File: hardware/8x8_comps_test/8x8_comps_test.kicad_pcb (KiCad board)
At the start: 2 copper layers, 47.8 x 47.5 mm, 24 parts

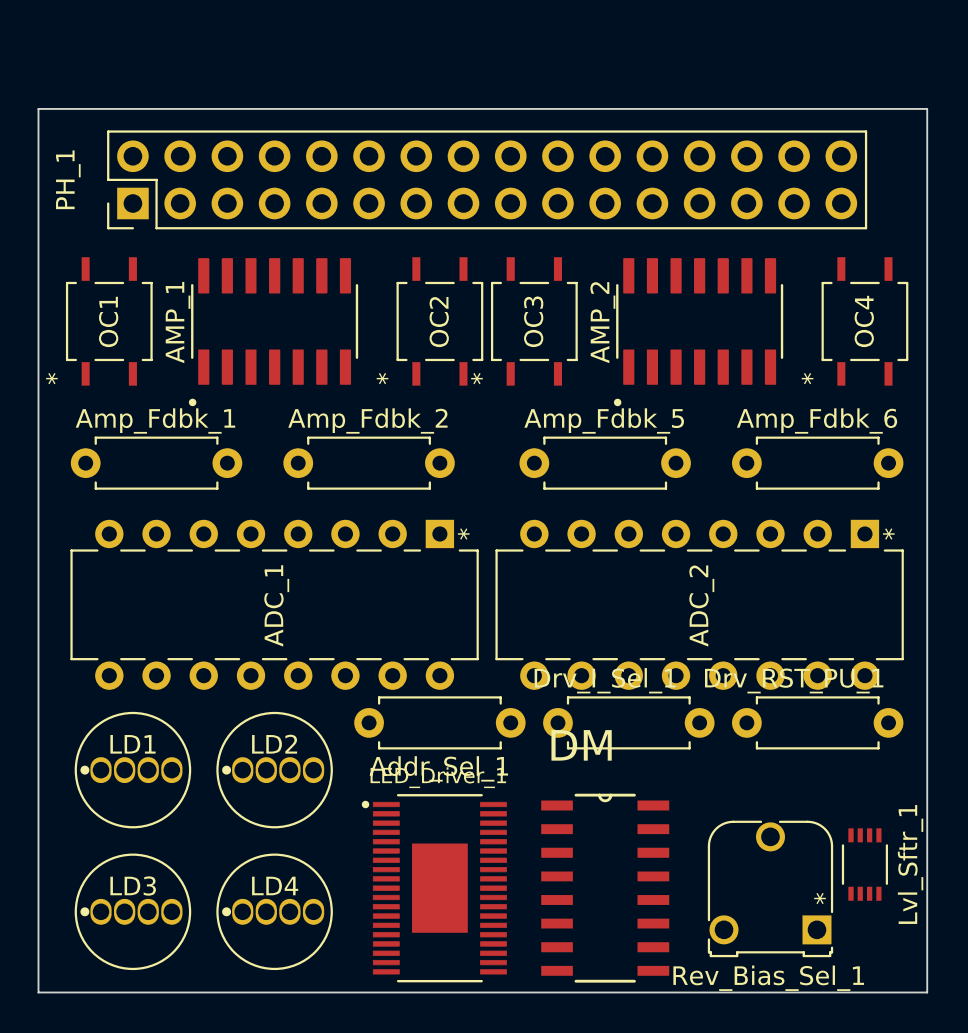
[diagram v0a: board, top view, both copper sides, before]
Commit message: Changed Test Layout
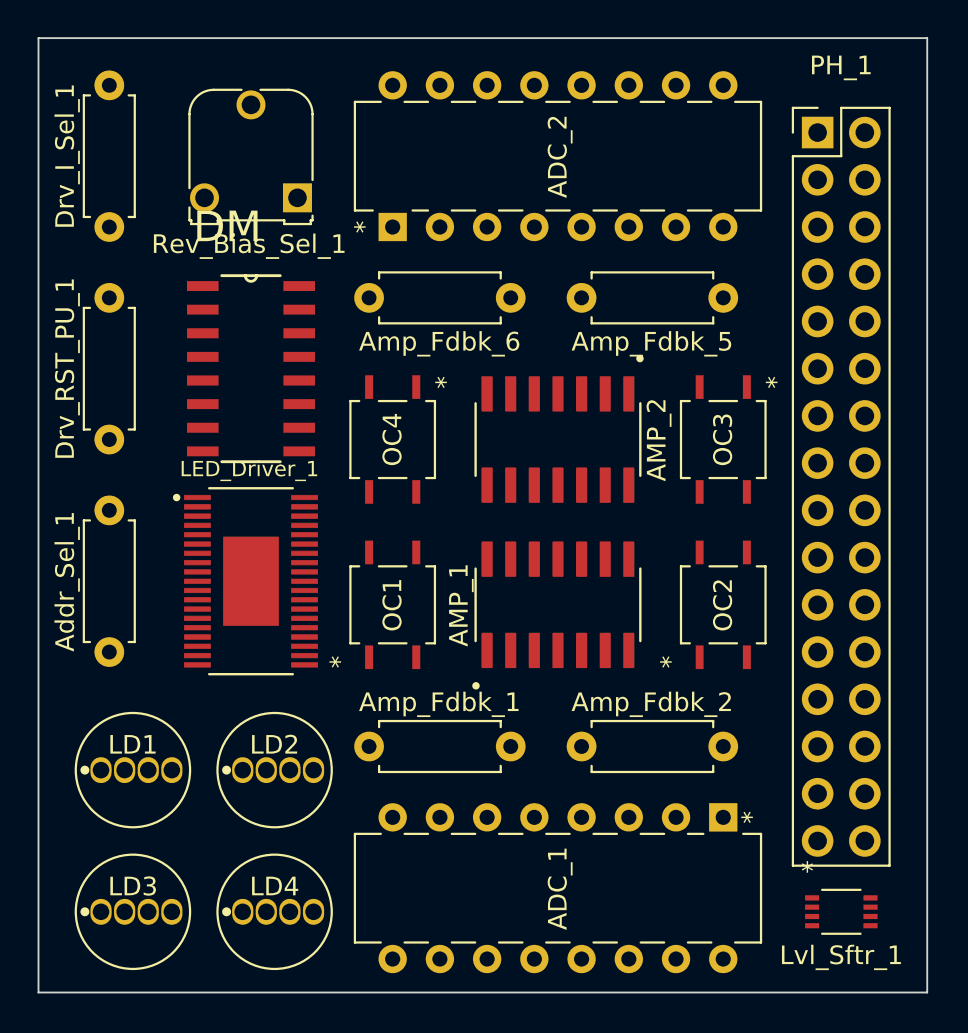
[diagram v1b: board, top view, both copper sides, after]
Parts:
- moved Rev_Bias_Sel_1 48.3 mm to (50.8, 37.8)
- moved Drv_RST_PU_1 37.5 mm to (40.6, 50.8), turned to 90 degrees
- moved PH_1 37.0 mm to (78.7, 34.3), turned to 0 degrees
- moved Drv_I_Sel_1 36.0 mm to (40.6, 39.4), turned to 90 degrees
- moved DM 33.8 mm to (48.3, 47.0)
- moved OC4 26.2 mm to (55.9, 50.8), turned to -90 degrees
- moved ADC_2 25.3 mm to (64.8, 35.6), turned to 90 degrees
- moved Addr_Sel_1 21.9 mm to (40.6, 62.2), turned to 90 degrees
- moved ADC_1 21.6 mm to (64.8, 74.9)
- moved Amp_Fdbk_1 21.6 mm to (54.6, 67.3)
- moved Amp_Fdbk_2 21.6 mm to (66.0, 67.3)
- moved OC1 21.6 mm to (55.9, 59.7)
- moved AMP_1 21.6 mm to (64.8, 59.7)
- moved OC2 21.6 mm to (73.7, 59.7)
- moved LED_Driver_1 19.4 mm to (48.3, 58.4)
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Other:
- board size 47.8 x 47.5 mm -> 47.8 x 51.3 mm

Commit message: Updated Components
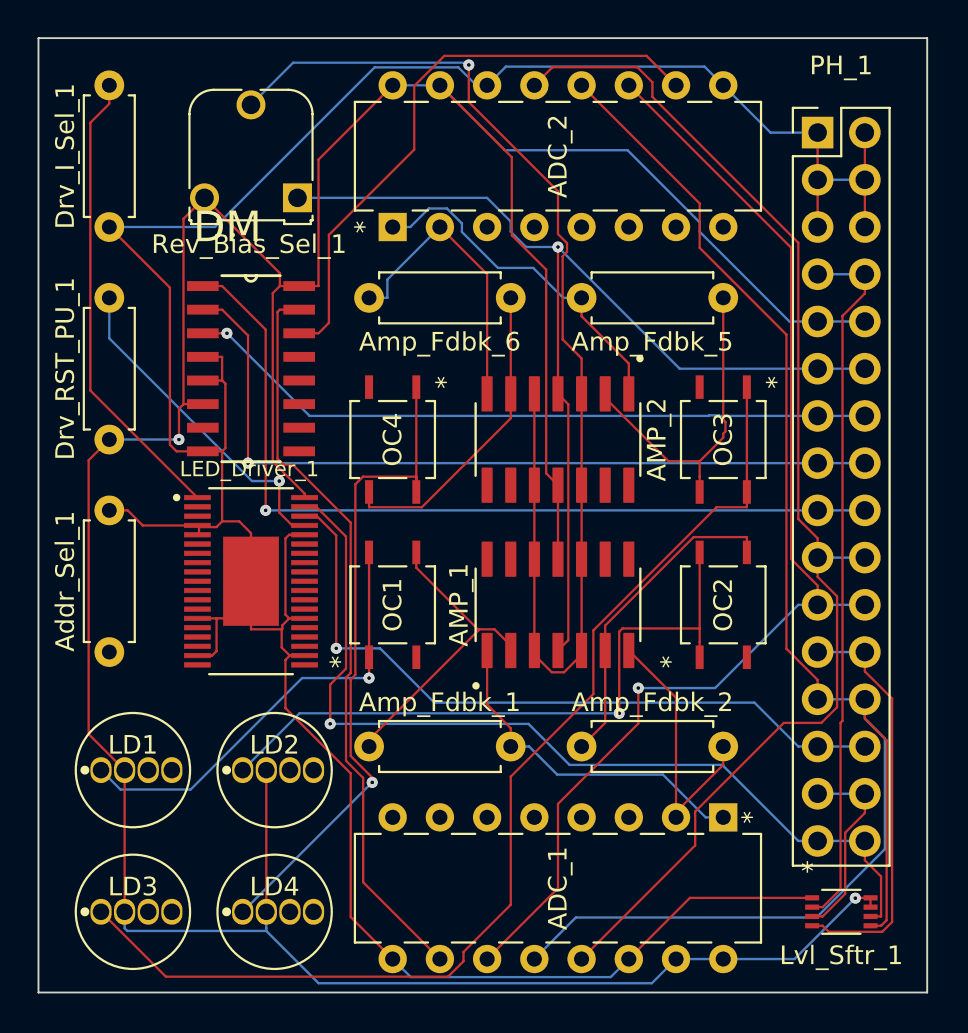
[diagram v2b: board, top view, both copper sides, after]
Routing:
- net +5V: track 0.00 -> 190.6 mm, vias 0 -> 2
- net GND: track 0.00 -> 158.2 mm
- net SPI_MISO_5V: track 0.00 -> 84.0 mm
- net SPI_SCK: track 0.00 -> 67.8 mm
- net RB Voltage: track 0.00 -> 64.5 mm, vias 0 -> 1
- net SPI_MOSI: track 0.00 -> 64.1 mm, vias 0 -> 1
- net /LED Row IO 2/LDRow/LD1_R: track 0.00 -> 59.4 mm
- net +9V: track 0.00 -> 56.8 mm, vias 0 -> 1
- net I2C_SDA_5V: track 0.00 -> 49.7 mm, vias 0 -> 1
- net SPI_SS_0: track 0.00 -> 46.3 mm, vias 0 -> 1
- net SPI_SS_1: track 0.00 -> 43.0 mm, vias 0 -> 1
- net /LED Row IO 1/ADC_SHDN: track 0.00 -> 40.1 mm
- net I2C_SCL: track 0.00 -> 38.8 mm, vias 0 -> 1
- net +3V3: track 0.00 -> 38.1 mm
- net SPI_SS_2: track 0.00 -> 37.5 mm, vias 0 -> 1
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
